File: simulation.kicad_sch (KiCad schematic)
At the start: 17 parts, among them U10 ${SIM.PARAMS}, U11 ${SIM.PARAMS}, U12 ${SIM.PARAMS}, U9 ${SIM.PARAMS}

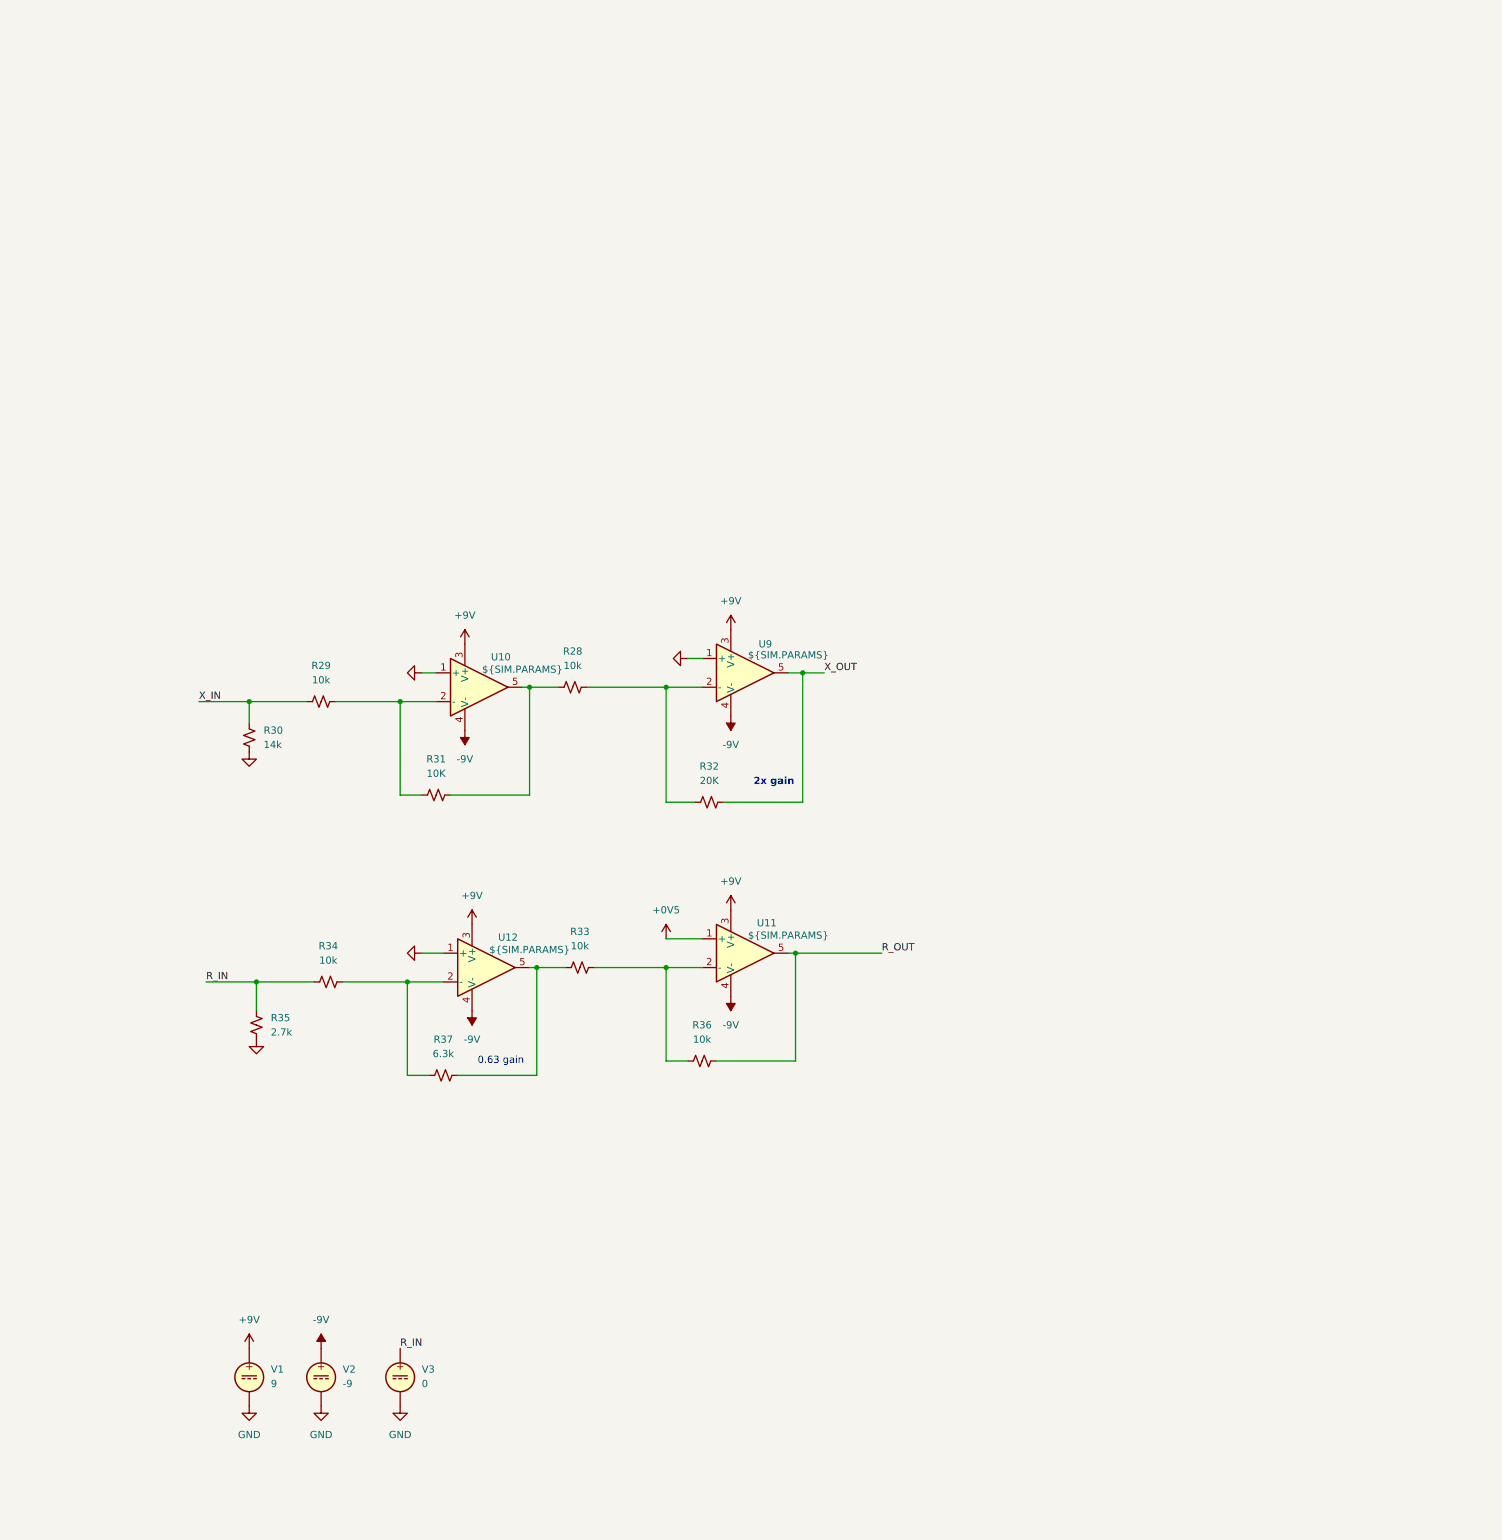
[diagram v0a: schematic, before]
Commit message: Add files via upload
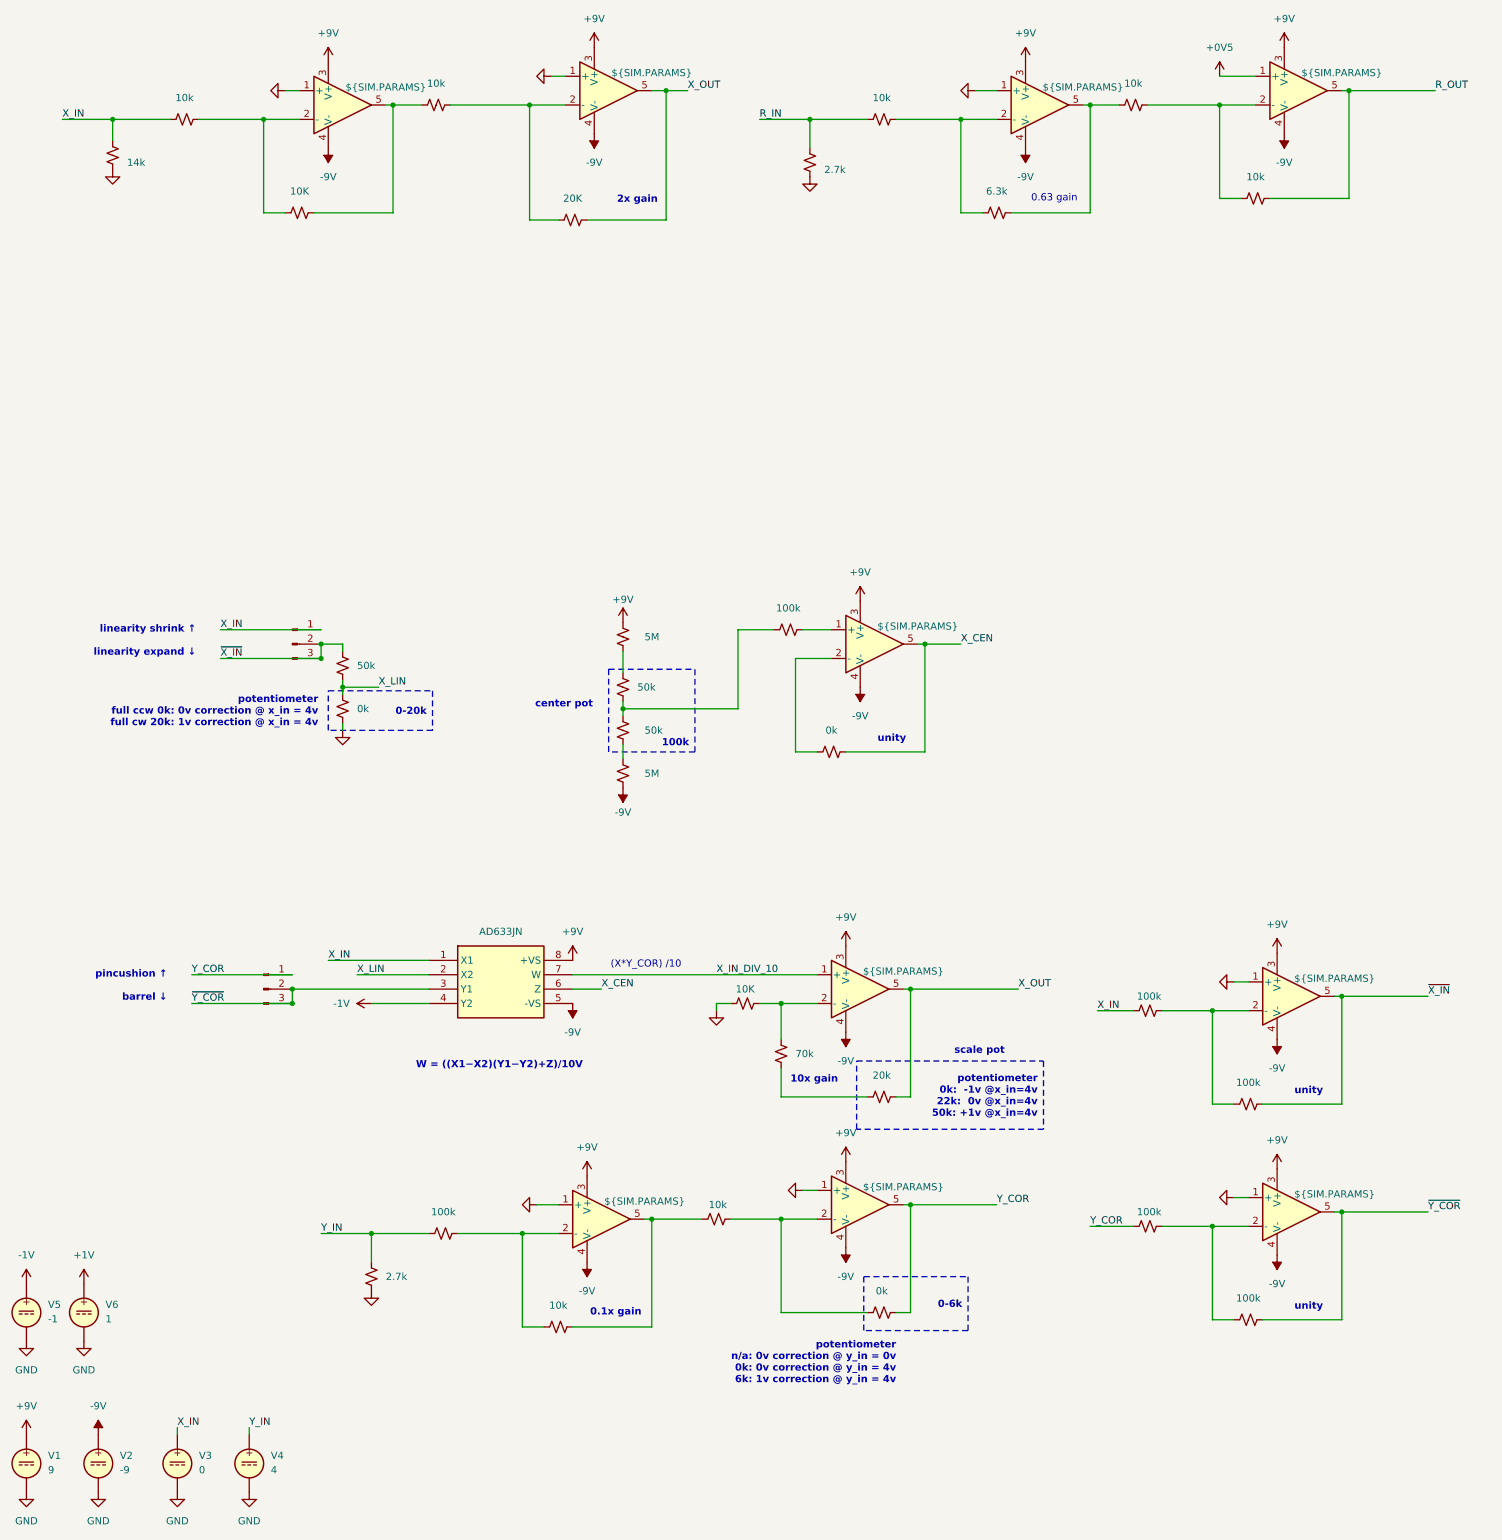
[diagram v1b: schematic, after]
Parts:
- added IC1: AD633JN, Package_DIP:DIP-8_W7.62mm_Socket, symbol AD633JN:AD633JN
- added J5, J6: Conn_01x03_Male, Connector_PinHeader_2.54mm:PinHeader_1x03_P2.54mm_Vertical, symbol Connector:Conn_01x03_Male
- added R38: 10K, Resistor_THT:R_Axial_DIN0207_L6.3mm_D2.5mm_P10.16mm_Horizontal, symbol Device:R_Small_US
- added R39, R44: 10k, Resistor_THT:R_Axial_DIN0207_L6.3mm_D2.5mm_P10.16mm_Horizontal, symbol Device:R_Small_US
- added R40, R45, R46, R49, R50, R53: 100k, Resistor_THT:R_Axial_DIN0207_L6.3mm_D2.5mm_P10.16mm_Horizontal, symbol Device:R_Small_US
- added R41: 20k, Resistor_THT:R_Axial_DIN0207_L6.3mm_D2.5mm_P10.16mm_Horizontal, symbol Device:R_Small_US
- added R42: 2.7k, Resistor_THT:R_Axial_DIN0207_L6.3mm_D2.5mm_P10.16mm_Horizontal, symbol Device:R_Small_US
- added R43, R47, R54: 0k, Resistor_THT:R_Axial_DIN0207_L6.3mm_D2.5mm_P10.16mm_Horizontal, symbol Device:R_Small_US
- added R48, R51, R52: 50k, Resistor_THT:R_Axial_DIN0207_L6.3mm_D2.5mm_P10.16mm_Horizontal, symbol Device:R_Small_US
- added R55: 70k, Resistor_THT:R_Axial_DIN0207_L6.3mm_D2.5mm_P10.16mm_Horizontal, symbol Device:R_Small_US
- added R57, R60: 5M, Resistor_THT:R_Axial_DIN0207_L6.3mm_D2.5mm_P10.16mm_Horizontal, symbol Device:R_Small_US
- added U13, U14, U15, U16, U17, U18: ${SIM.PARAMS}, symbol Simulation_SPICE:OPAMP
- added V4: 4, symbol Simulation_SPICE:VDC
- added V5: -1, symbol Simulation_SPICE:VDC
- added V6: 1, symbol Simulation_SPICE:VDC
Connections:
- net +9V: now also IC1.8 (+VS), R57.2, U13.3 (V+), U14.3 (V+), U15.3 (V+), U16.3 (V+), U17.3 (V+), U18.3 (V+)
- net -9V: now also IC1.5 (-VS), R60.1, U13.4 (V-), U14.4 (V-), U15.4 (V-), U16.4 (V-), U17.4 (V-), U18.4 (V-)
- net GND: now also R38.1, R42.1, R47.1, U13.1 (+), U15.1 (+), U16.1 (+), U17.1 (+), V4.2, V5.2, V6.2
- net R_IN: no longer V3.1
- net X_IN: now also V3.1, IC1.1 (X1), J6.1 (Pin_1), R49.1
- net X_OUT: now also R41.2, U14.5
- new net: R51.1, R52.2, R53.1
- new net: R51.2, R57.1
- new net: R38.2, R55.2, U14.2 (-)
- new net: R41.1, R55.1
- new net: R40.2, R44.1, U15.2 (-)
- new net: R39.1, R44.2, U15.5
- new net: R53.2, U18.1 (+)
- new net: R54.1, U18.2 (-)
- new net: R52.1, R60.2
- new net: R49.2, R50.1, U17.2 (-)
- new net: R45.2, R46.1, U16.2 (-)
- new net: R39.2, R43.1, U13.2 (-)
- new net +1V: V6.1
- new net -1V: IC1.4 (Y2), V5.1
- new net X_CEN: IC1.6 (Z), R54.2, U18.5
- new net X_IN_DIV_10: IC1.7 (W), U14.1 (+)
- new net X_LIN: IC1.2 (X2), R47.2, R48.1
- new net Y_COR: J5.1 (Pin_1), R43.2, R45.1, U13.5
- new net Y_IN: R40.1, R42.2, V4.1
- new net ~{X_IN}: J6.2 (Pin_2), J6.3 (Pin_3), R48.2, R50.2, U17.5
- new net ~{Y_COR}: IC1.3 (Y1), J5.2 (Pin_2), J5.3 (Pin_3), R46.2, U16.5
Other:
- note added: "(X*Y_COR) /10"
- note added: "0.1x gain"
- note added: "10x gain"
- note added: "W = ((X1−X2)(Y1−Y2)+Z)/10V"
- note added: "center pot"
- note added: "linearity shrink ↑ linearity expand ↓"
- note added: "pincushion ↑ barrel ↓"
- note added: "potentiometer full ccw 0k: 0v correction @ x_in = 4v full cw 20k: 1v correction @ x_in = 4v"
- note added: "potentiometer n/a: 0v correction @ y_in = 0v 0k: 0v correction @ y_in = 4v 6k: 1v correction @ y_in = 4v"
- note added: "scale pot"
- note added: "unity"
- moved on the sheet: V1, V2, V3
